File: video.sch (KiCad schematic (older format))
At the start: 32 parts, among them CN10 COMPOSITE, CN9 VIDEO_DB23M, U4 DENISE, U40 74LS245, U41 74LS245

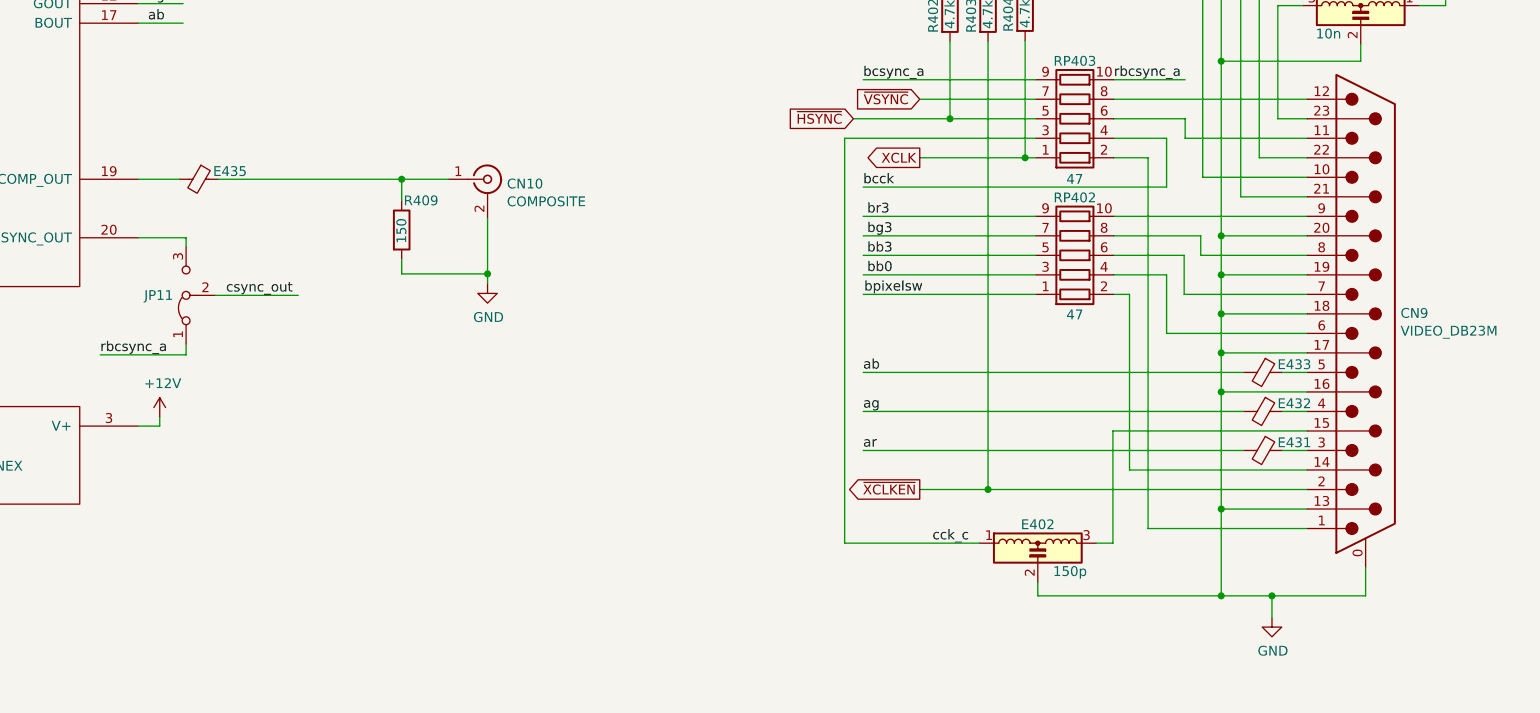
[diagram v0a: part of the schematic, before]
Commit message: Work in progress
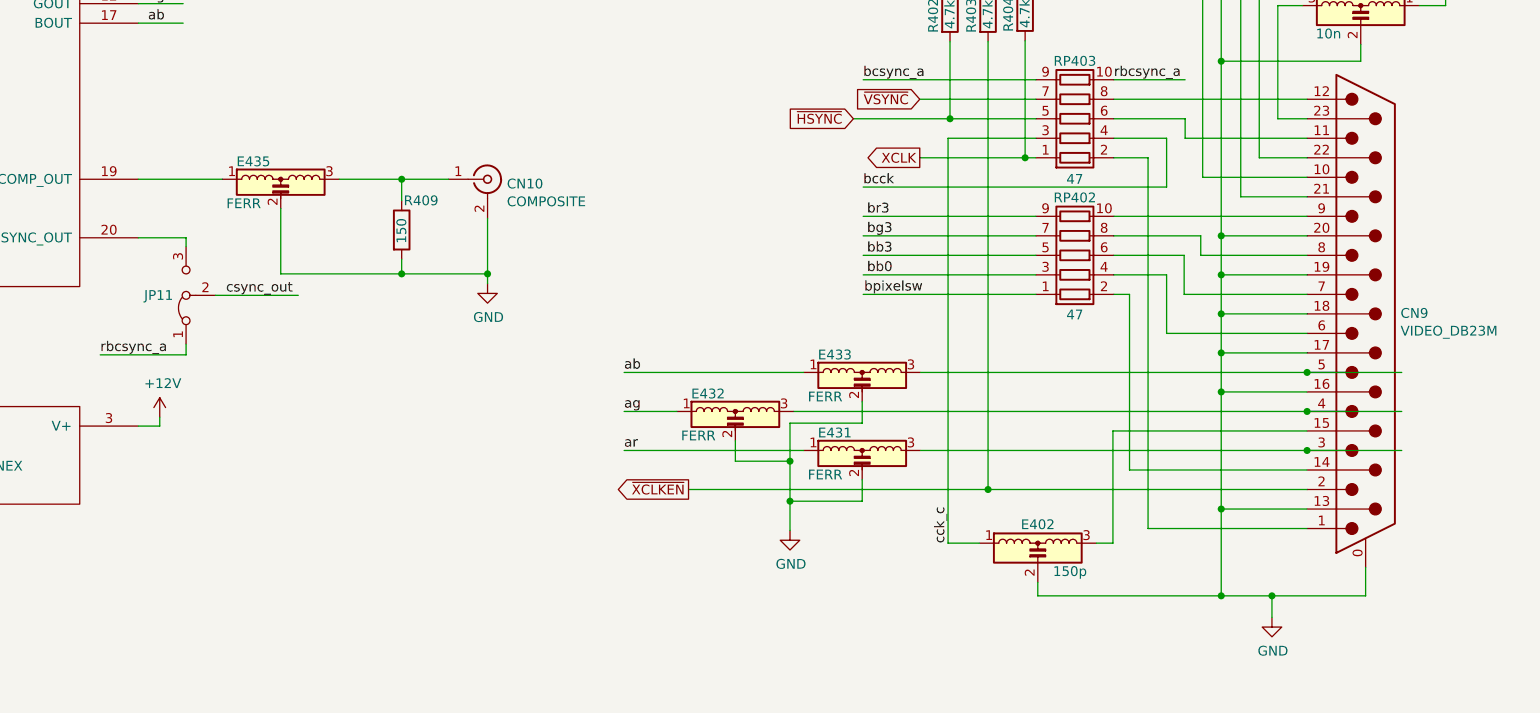
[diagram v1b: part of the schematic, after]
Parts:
- removed E431, E432, E433, E435: Ferrite_Bead_Small, Raemixx500:EMI_Filter_Long, symbol Device:Ferrite_Bead_Small
- added E431, E432, E433, E435: FERR, Raemixx500:EMI_Filter_Long, symbol emi_filter_lcl_small:EMI_Filter_LCL
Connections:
- wire segments 300 -> 314
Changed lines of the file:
@@
 Wire Wire Line
 	14380 5565 12745 5565
-Text GLabel 12395 5565 0    50   Output ~ 0
-~XCLKEN
 Wire Wire Line
 	6030 3975 6690 3975
@@
 Wire Wire Line
 	13940 4265 13940 4465
-$Comp
-L Device:Ferrite_Bead_Small E433
-U 1 1 5CFAFD37
-P 14155 4965
-F 0 "E433" V 14115 5125 50  0000 C CNN
-F 1 "Ferrite_Bead_Small" V 14009 4965 50  0001 C CNN
-F 2 "Raemixx500:EMI_Filter_Long" V 14085 4965 50  0001 C CNN
-F 3 "~" H 14155 4965 50  0001 C CNN
-	1    14155 4965
-	0    1    1    0
-$EndComp
-$Comp
-L Device:Ferrite_Bead_Small E432
-U 1 1 5CFAFFD0
-P 14155 5165
-F 0 "E432" V 14115 5325 50  0000 C CNN
-F 1 "Ferrite_Bead_Small" V 14009 5165 50  0001 C CNN
-F 2 "Raemixx500:EMI_Filter_Long" V 14085 5165 50  0001 C CNN
-F 3 "~" H 14155 5165 50  0001 C CNN
-	1    14155 5165
-	0    1    1    0
-$EndComp
-$Comp
-L Device:Ferrite_Bead_Small E431
-U 1 1 5CFB0114
-P 14155 5365
-F 0 "E431" V 14115 5525 50  0000 C CNN
-F 1 "Ferrite_Bead_Small" V 14009 5365 50  0001 C CNN
-F 2 "Raemixx500:EMI_Filter_Long" V 14085 5365 50  0001 C CNN
-F 3 "~" H 14155 5365 50  0001 C CNN
-	1    14155 5365
-	0    1    1    0
-$EndComp
-Wire Wire Line
-	14255 4965 14380 4965
-Wire Wire Line
-	14255 5165 14380 5165
-Wire Wire Line
-	14255 5365 14380 5365
-Wire Wire Line
-	14055 4965 12105 4965
-Wire Wire Line
-	14055 5165 12105 5165
-Wire Wire Line
-	14055 5365 12105 5365
-Text Label 12105 4965 0    50   ~ 0
+Text Label 10880 4965 0    50   ~ 0
 ab
-Text Label 12105 5165 0    50   ~ 0
+Text Label 10880 5165 0    50   ~ 0
 ag
-Text Label 12105 5365 0    50   ~ 0
+Text Label 10880 5365 0    50   ~ 0
 ar
 Wire Wire Line
@@
 	13385 5265 13385 5840
 Wire Wire Line
-	12990 3765 12010 3765
-Wire Wire Line
-	12010 3765 12010 5840
-Wire Wire Line
-	12010 5840 12700 5840
-Text Label 12460 5840 0    50   ~ 0
+	12990 3765 12540 3765
+Wire Wire Line
+	12540 3765 12540 5840
+Wire Wire Line
+	12540 5840 12700 5840
+Text Label 12540 5840 1    50   ~ 0
 cck_c
 $Comp
@@
 Connection ~ 12745 5565
 Wire Wire Line
-	12745 5565 12395 5565
+	12745 5565 11210 5565
 Wire Wire Line
 	12550 2970 12550 2835
@@
 rbcsync_a
 $Comp
-L Device:Ferrite_Bead_Small E435
-U 1 1 5D99AF23
-P 8700 3975
-F 0 "E435" V 8660 4135 50  0000 C CNN
-F 1 "Ferrite_Bead_Small" V 8554 3975 50  0001 C CNN
-F 2 "Raemixx500:EMI_Filter_Long" V 8630 3975 50  0001 C CNN
-F 3 "~" H 8700 3975 50  0001 C CNN
-	1    8700 3975
-	0    1    1    0
-$EndComp
-$Comp
 L Connector:Conn_Coaxial CN?
 U 1 1 5D9B0BDD
@@
 	1    0    0    -1
 $EndComp
-Wire Wire Line
-	8800 3975 9740 3975
 $Comp
 L power:GND #PWR0264
@@
 Wire Wire Line
 	9740 4385 9740 4460
-Wire Wire Line
-	9740 4460 10180 4460
 Connection ~ 10180 4460
 Wire Wire Line
@@
 Wire Wire Line
 	13460 2965 13940 2965
-Wire Wire Line
-	8390 3975 8600 3975
 $Comp
 L VIDIOT:VIDIOT_ANNEX HY2
@@
 Wire Wire Line
 	8500 5240 8500 5195
+$Comp
+L emi_filter_lcl_small:EMI_Filter_LCL E?
+U 1 1 5DD342FD
+P 12100 5065
+AR Path="/5E7E9EC4/5DD342FD" Ref="E?"  Part="1"
+AR Path="/5CBA5669/5DD342FD" Ref="E433"  Part="1"
+F 0 "E433" H 11960 5255 50  0000 C CNN
+F 1 "FERR" H 11910 5040 50  0000 C CNN
+F 2 "Raemixx500:EMI_Filter_Long" V 12100 5065 50  0001 C CNN
+F 3 "http://www.murata.com/~/media/webrenewal/support/library/catalog/products/emc/emifil/c31e.ashx?la=en-gb" V 12100 5065 50  0001 C CNN
+	1    12100 5065
+	1    0    0    -1
+$EndComp
+$Comp
+L emi_filter_lcl_small:EMI_Filter_LCL E?
+U 1 1 5DD4BEEC
+P 12100 5465
+AR Path="/5E7E9EC4/5DD4BEEC" Ref="E?"  Part="1"
+AR Path="/5CBA5669/5DD4BEEC" Ref="E431"  Part="1"
+F 0 "E431" H 11960 5655 50  0000 C CNN
+F 1 "FERR" H 11910 5440 50  0000 C CNN
+F 2 "Raemixx500:EMI_Filter_Long" V 12100 5465 50  0001 C CNN
+F 3 "http://www.murata.com/~/media/webrenewal/support/library/catalog/products/emc/emifil/c31e.ashx?la=en-gb" V 12100 5465 50  0001 C CNN
+	1    12100 5465
+	1    0    0    -1
+$EndComp
+$Comp
+L emi_filter_lcl_small:EMI_Filter_LCL E?
+U 1 1 5DD7EF86
+P 11450 5265
+AR Path="/5E7E9EC4/5DD7EF86" Ref="E?"  Part="1"
+AR Path="/5CBA5669/5DD7EF86" Ref="E432"  Part="1"
+F 0 "E432" H 11310 5455 50  0000 C CNN
+F 1 "FERR" H 11260 5240 50  0000 C CNN
+F 2 "Raemixx500:EMI_Filter_Long" V 11450 5265 50  0001 C CNN
+F 3 "http://www.murata.com/~/media/webrenewal/support/library/catalog/products/emc/emifil/c31e.ashx?la=en-gb" V 11450 5265 50  0001 C CNN
+	1    11450 5265
+	1    0    0    -1
+$EndComp
+Wire Wire Line
+	11800 4965 10880 4965
+Wire Wire Line
+	11150 5165 10880 5165
+Wire Wire Line
+	11800 5365 10880 5365
+Wire Wire Line
+	12400 4965 14380 4965
+Wire Wire Line
+	11750 5165 14380 5165
+Wire Wire Line
+	12400 5365 14380 5365
+Text GLabel 11210 5565 0    50   Output ~ 0
+~XCLKEN
+Connection ~ 14380 4965
+Wire Wire Line
+	14380 4965 14865 4965
+Connection ~ 14380 5165
+Wire Wire Line
+	14380 5165 14865 5165
+Connection ~ 14380 5365
+Wire Wire Line
+	14380 5365 14865 5365
+Wire Wire Line
+	12100 5115 12100 5225
+Wire Wire Line
+	12100 5225 11730 5225
+Wire Wire Line
+	11730 5225 11730 5420
+Wire Wire Line
+	11450 5315 11450 5420
+Wire Wire Line
+	11450 5420 11730 5420
+Connection ~ 11730 5420
+Wire Wire Line
+	11730 5420 11730 5625
+Wire Wire Line
+	12100 5515 12100 5625
+Wire Wire Line
+	12100 5625 11730 5625
+Connection ~ 11730 5625
+Wire Wire Line
+	11730 5625 11730 5775
+$Comp
+L power:GND #PWR0269
+U 1 1 5DF44B74
+P 11730 5775
+F 0 "#PWR0269" H 11730 5525 50  0001 C CNN
+F 1 "GND" H 11735 5602 50  0000 C CNN
+F 2 "" H 11730 5775 50  0001 C CNN
+F 3 "" H 11730 5775 50  0001 C CNN
+	1    11730 5775
+	1    0    0    -1
+$EndComp
+Wire Wire Line
+	8390 3975 8820 3975
+Wire Wire Line
+	9420 3975 9740 3975
+$Comp
+L emi_filter_lcl_small:EMI_Filter_LCL E?
+U 1 1 5DF6B27A
+P 9120 4075
+AR Path="/5E7E9EC4/5DF6B27A" Ref="E?"  Part="1"
+AR Path="/5CBA5669/5DF6B27A" Ref="E435"  Part="1"
+F 0 "E435" H 8980 4265 50  0000 C CNN
+F 1 "FERR" H 8930 4050 50  0000 C CNN
+F 2 "Raemixx500:EMI_Filter_Long" V 9120 4075 50  0001 C CNN
+F 3 "http://www.murata.com/~/media/webrenewal/support/library/catalog/products/emc/emifil/c31e.ashx?la=en-gb" V 9120 4075 50  0001 C CNN
+	1    9120 4075
+	1    0    0    -1
+$EndComp
+Wire Wire Line
+	9120 4125 9120 4460
+Wire Wire Line
+	9120 4460 9740 4460
 Wire Bus Line
 	2005 3775 2005 4475
 Wire Bus Line
 	2005 2075 2005 3575
+Connection ~ 9740 4460
+Wire Wire Line
+	9740 4460 10180 4460
 $EndSCHEMATC
